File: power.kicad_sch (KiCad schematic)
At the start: 32 parts, among them J4 USB_C_Receptacle_USB2.0_16P, U1 TPS62840DLC, U2 BQ25170DSGR, U3 LM66100DCK, U6 LM66100DCK

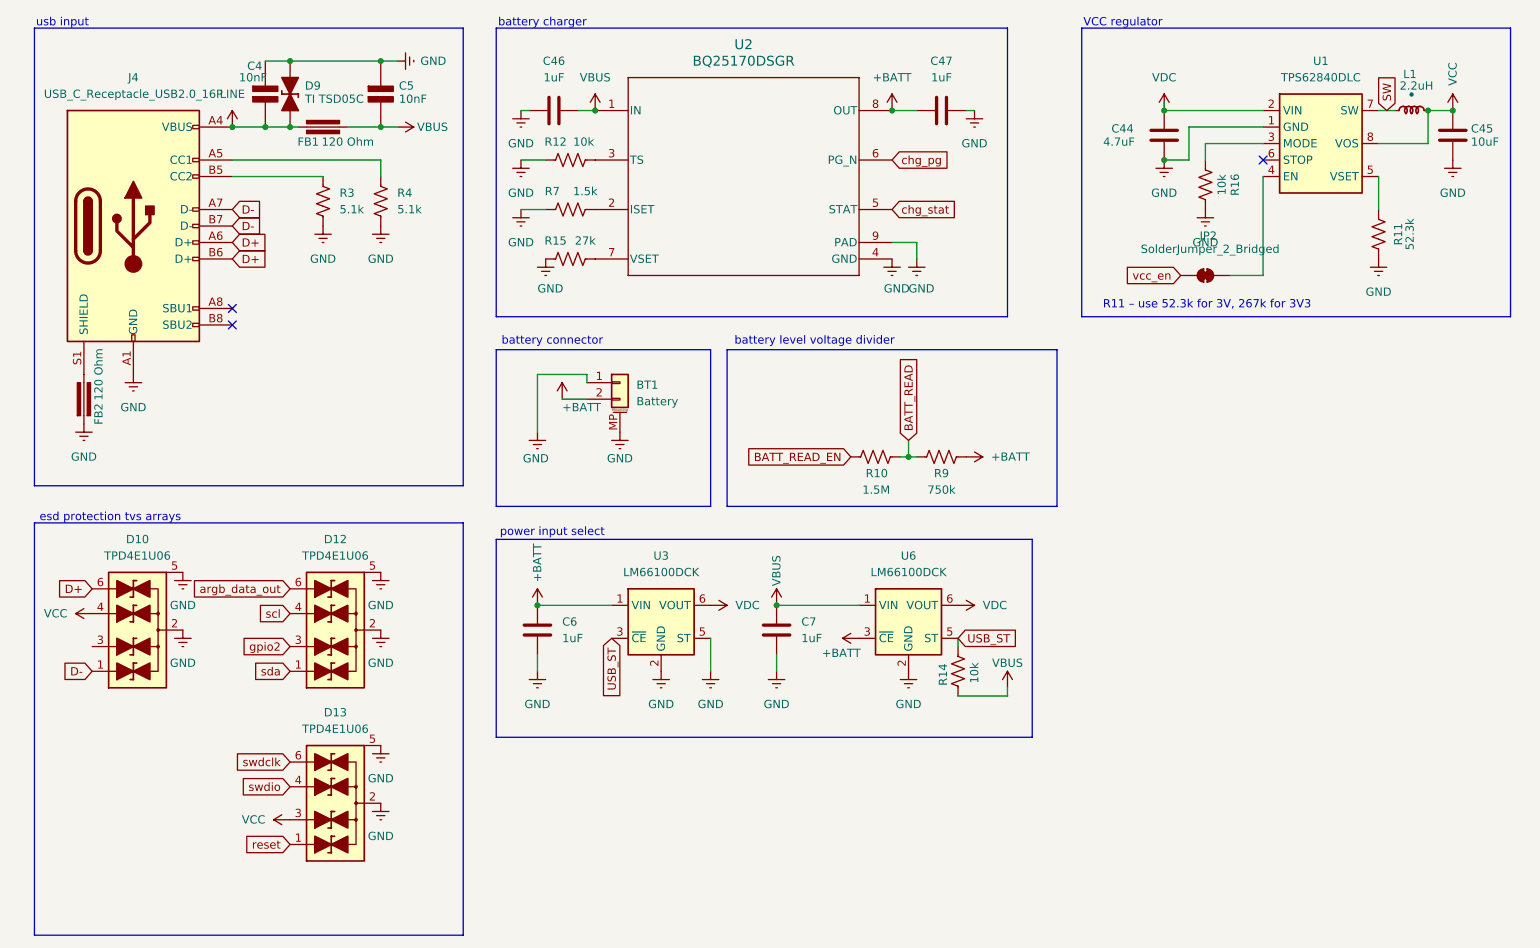
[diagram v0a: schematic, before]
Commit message: progress
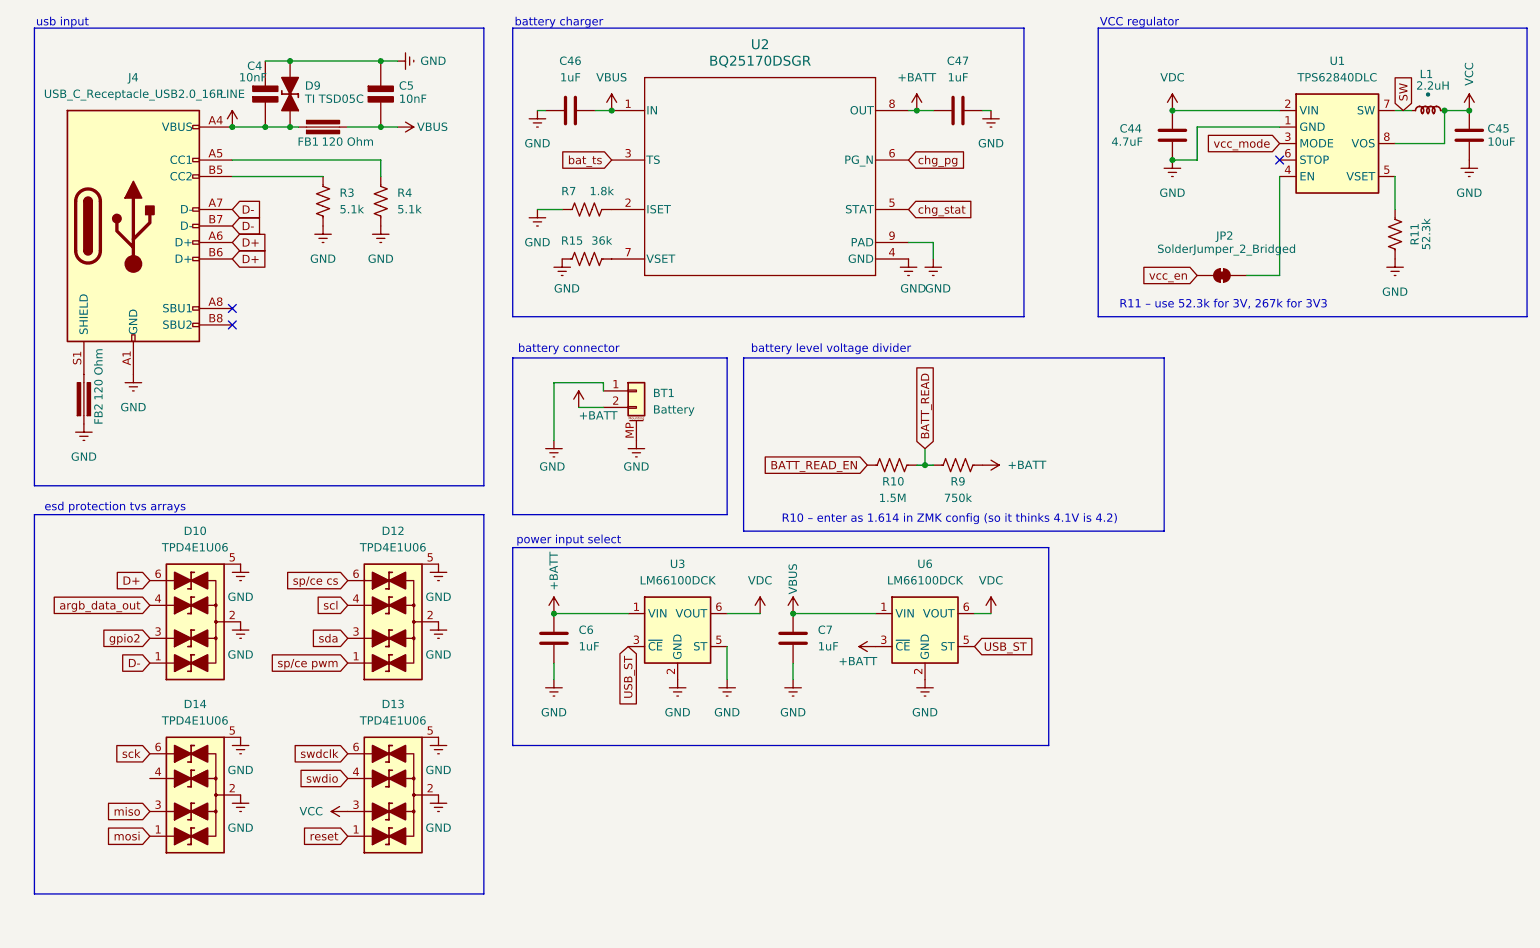
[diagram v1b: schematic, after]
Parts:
- removed R12, R14, R16: 10k, Resistor_SMD:R_0603_1608Metric, symbol Device:R_US
- added D14: TPD4E1U06, coquette_footprints:TPD4E1U06, symbol coquette_symbols:TPD4E1U06
- R15: value 27k -> 36k
- R7: value 1.5k -> 1.8k
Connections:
- net GND: now also D14.2 (VN), D14.5 (NC)
- net VCC: no longer D10.4 (L3)
- net argb_data_out: now also D10.4 (L3); no longer D12.6 (L4)
- net gpio2: now also D10.3 (L2); no longer D12.3 (L2)
- net sda: now also D12.3 (L2); no longer D12.1 (L1)
- net bat_ts: now reaches U2.3 (TS)
- net vcc_mode: now reaches U1.3 (MODE)
- new net miso: D14.3 (L2)
- new net mosi: D14.1 (L1)
- new net sck: D14.6 (L4)
- new net sp/ce cs: D12.6 (L4)
- new net sp/ce pwm: D12.1 (L1)
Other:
- note added: "R10 – enter as 1.614 in ZMK config (so it thinks 4.1V is 4.2)"
- moved on the sheet: BT1, C44, C45, C46, C47, C6, C7, D10, D12, D13, JP2, L1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

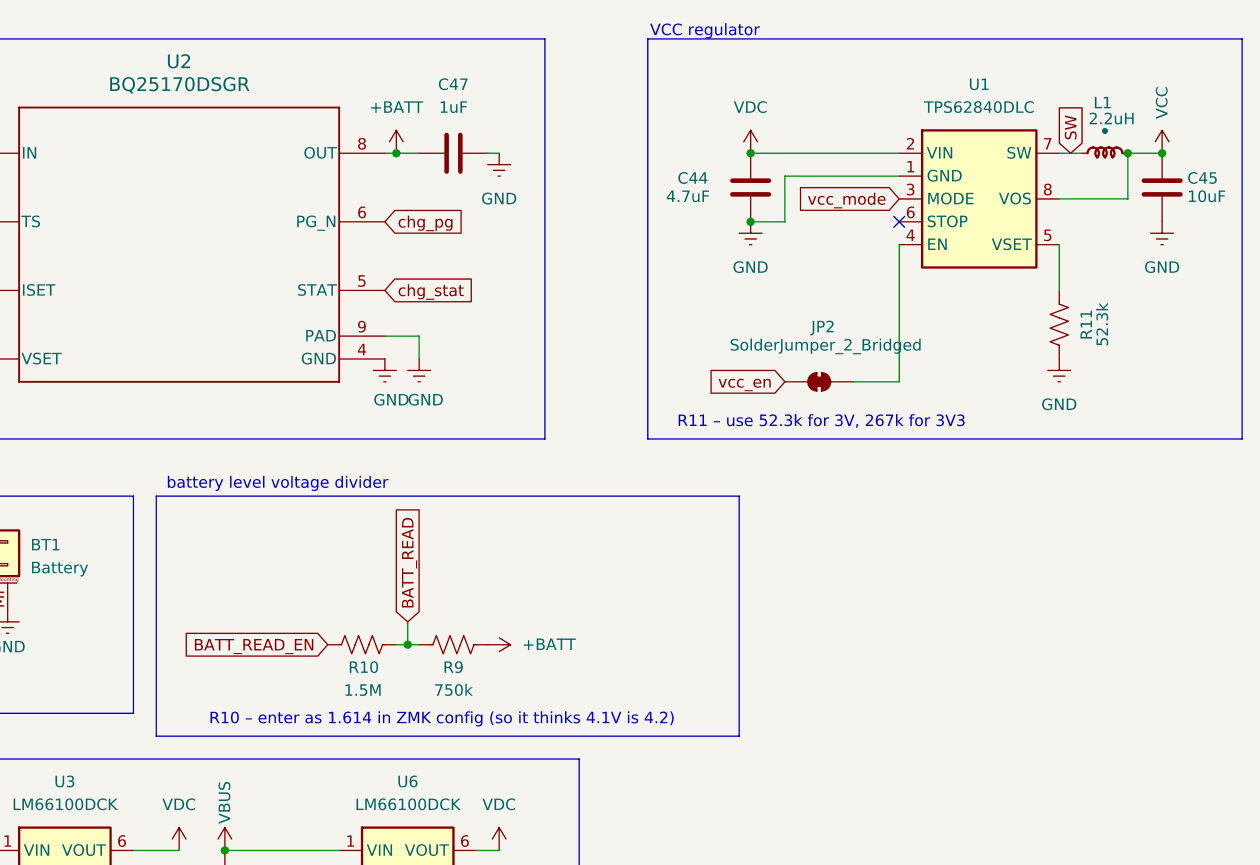
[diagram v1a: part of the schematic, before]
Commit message: new dcdc
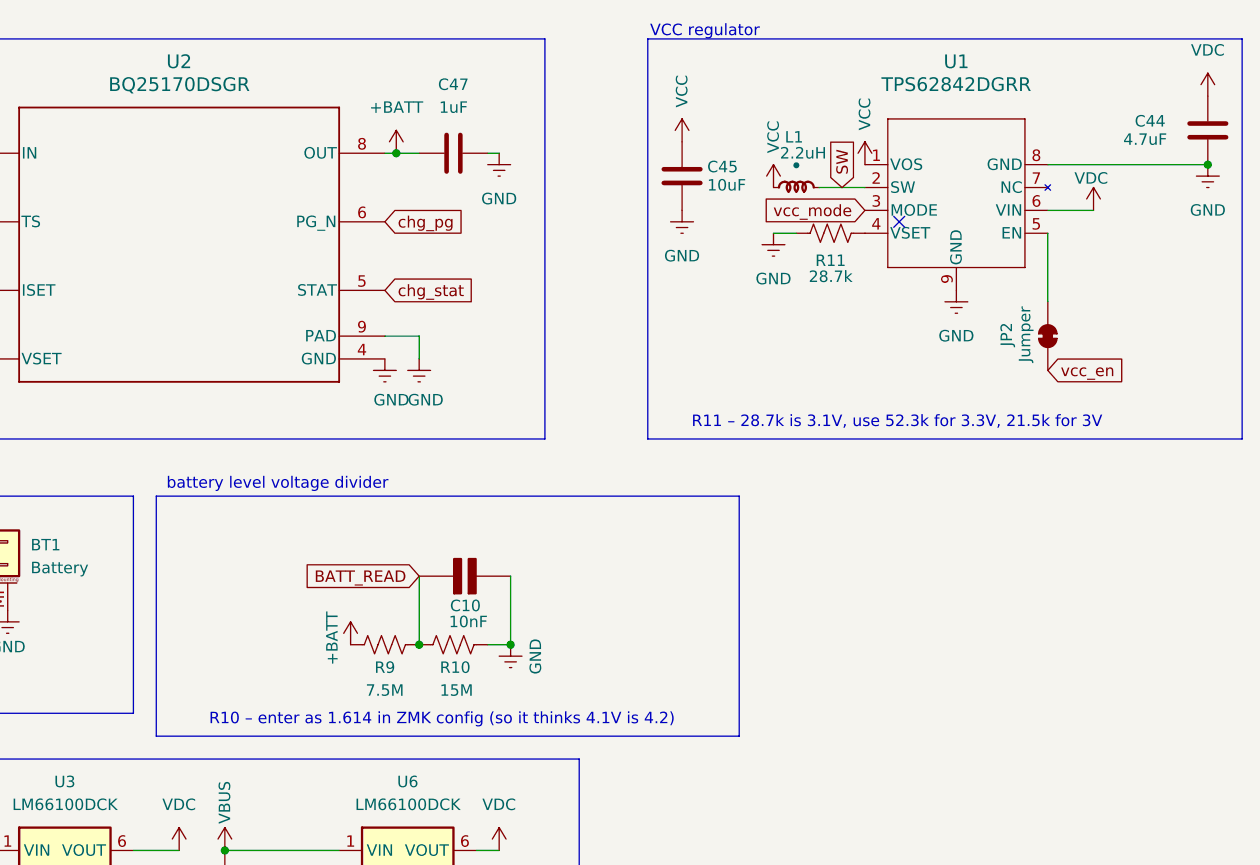
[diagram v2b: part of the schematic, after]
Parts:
- removed U1: TPS62840DLC, Package_SON:Texas_VSON-HR-8_1.5x2mm_P0.5mm, symbol coquette_symbols:TPS62840DLC
- added C10: 10nF, Capacitor_SMD:C_0603_1608Metric, symbol PCM_Elektuur:C
- added U1: TPS62842DGRR, Package_SO:HVSSOP-8-1EP_3x3mm_P0.65mm_EP1.57x1.89mm_ThermalVias, symbol mariposa:TPS62842DGRR
- JP2: value SolderJumper_2_Bridged -> Jumper
- R10: value 1.5M -> 15M; footprint Resistor_SMD:R_0603_1608Metric -> Resistor_SMD:R_1206_3216Metric
- R11: value 52.3k -> 28.7k
- R9: value 750k -> 7.5M
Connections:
- net BATT_READ_EN is gone; now on net BATT_READ: R10.2
- net +BATT: now also R9.2; no longer R9.1
- net BATT_READ: now also R9.1, C10.1 (+); no longer R10.1, R9.2
- net GND: now also R10.1, C10.2 (-), U1.8 (GND), U1.9 (GND)
- net SW: now also L1.2 (-), U1.2 (SW); no longer L1.1 (+)
- net VCC: now also L1.1 (+), U1.1 (VOS); no longer L1.2 (-)
- net VDC: now also U1.6 (VIN)
- net vcc_mode: now also U1.3 (MODE)
- net at JP2.1 (A): now also U1.5 (EN)
- net at R11.1: now also U1.4 (VSET)
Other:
- note added: "R11 – 28.7k is 3.1V, use 52.3k for 3.3V, 21.5k for 3V"
- note removed: "R11 – use 52.3k for 3V, 267k for 3V3"
- moved on the sheet: C44, C45, JP2, L1, R10, R11, R9

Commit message: tweaks
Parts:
- C44: footprint Capacitor_SMD:C_0603_1608Metric -> Capacitor_SMD:C_1206_3216Metric
- C45: footprint Capacitor_SMD:C_0603_1608Metric -> Capacitor_SMD:C_0805_2012Metric
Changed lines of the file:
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@@
 		(length 2.54)
 		(shape diamond)
-		(at 179.07 35.56 90)
-		(effects
-			(font
-				(size 1.27 1.27)
-			)
-			(justify left bottom)
-		)
-		(property "Netclass" "power"
-			(at 176.53 42.164 90)
-			(effects
-				(font
-					(size 1.27 1.27)
-					(italic yes)
-				)
-				(justify left)
-			)
-		)
-	)
-	(netclass_flag ""
-		(length 2.54)
-		(shape diamond)
 		(at 50.8 38.1 180)
 		(effects
@@
 			)
 		)
-		(property "Footprint" "Capacitor_SMD:C_0603_1608Metric"
+		(property "Footprint" "Capacitor_SMD:C_1206_3216Metric"
 			(at 247.3452 36.83 0)
 			(effects
@@
 			)
 		)
-		(property "Footprint" "Capacitor_SMD:C_0603_1608Metric"
+		(property "Footprint" "Capacitor_SMD:C_0805_2012Metric"
 			(at 188.9252 41.91 0)
 			(effects
